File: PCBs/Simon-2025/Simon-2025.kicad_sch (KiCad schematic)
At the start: 13 parts, among them IC1 MSPM0G3507SDGS28R, J1 Conn_01x09, J2 Conn_01x05, SW6 SW_SPDT, U1 LIS2HH12

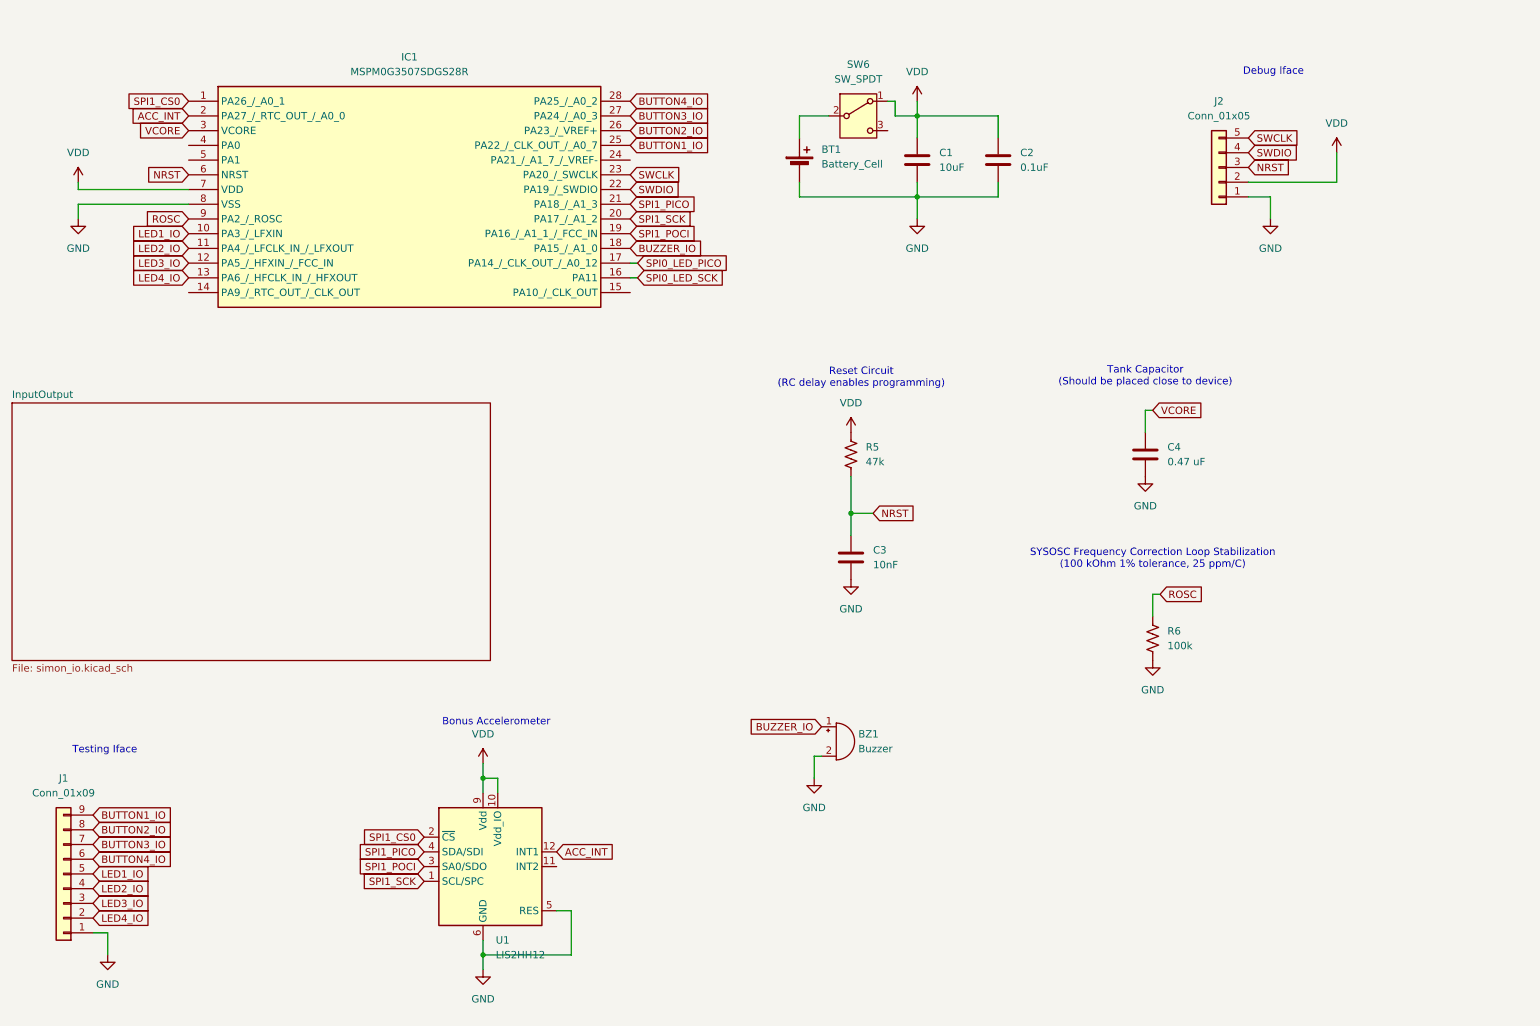
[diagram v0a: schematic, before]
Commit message: Updated Simon PCB 2025
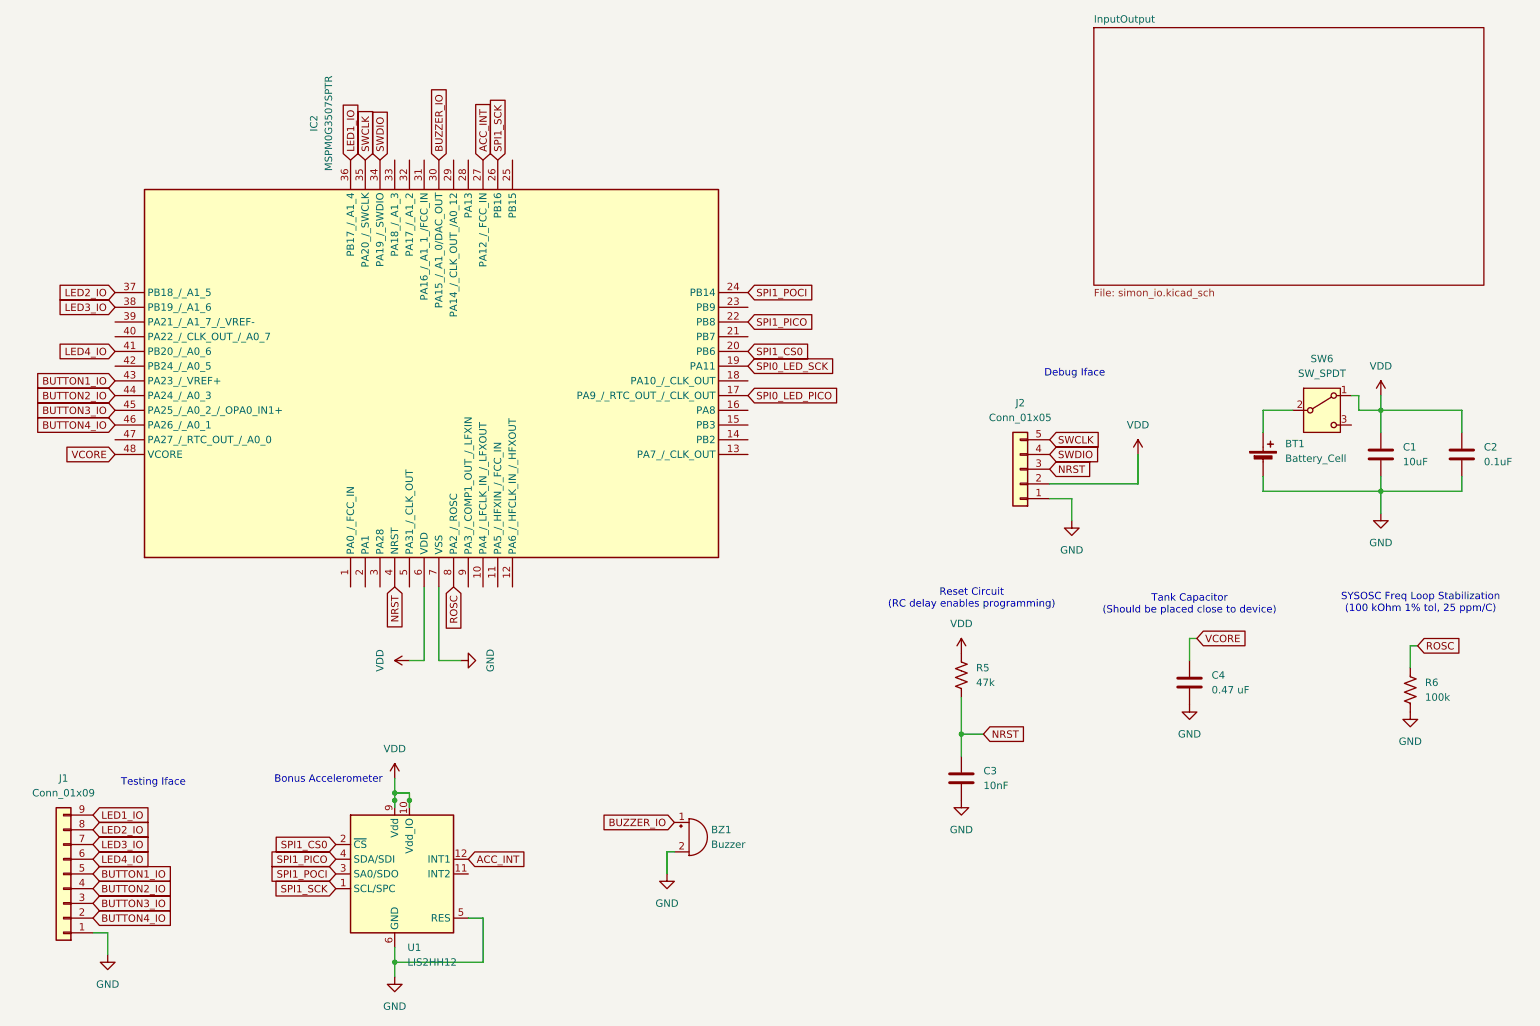
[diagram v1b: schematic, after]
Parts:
- removed IC1: MSPM0G3507SDGS28R, SOP50P490X110-28N, symbol ELEC327-Kicad:MSPM0G3507SDGS28R
- added IC2: MSPM0G3507SPTR, QFP50P900X900X160-48N, symbol ELEC327-Kicad:MSPM0G3507SPTR
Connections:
- net ACC_INT: now also IC2.27 (PA12_/_FCC_IN)
- net BUTTON1_IO: now also J1.5 (Pin_5), IC2.43 (PA23_/_VREF+); no longer J1.9 (Pin_9)
- net BUTTON2_IO: now also J1.4 (Pin_4), IC2.44 (PA24_/_A0_3); no longer J1.8 (Pin_8)
- net BUTTON3_IO: now also J1.3 (Pin_3), IC2.45 (PA25_/_A0_2_/_OPA0_IN1+); no longer J1.7 (Pin_7)
- net BUTTON4_IO: now also J1.2 (Pin_2), IC2.46 (PA26_/_A0_1); no longer J1.6 (Pin_6)
- net BUZZER_IO: now also IC2.30 (PA15_/_A1_0/DAC_OUT)
- net GND: now also IC2.7 (VSS)
- net LED1_IO: now also J1.9 (Pin_9), IC2.36 (PB17_/_A1_4); no longer J1.5 (Pin_5)
- net LED2_IO: now also J1.8 (Pin_8), IC2.37 (PB18_/_A1_5); no longer J1.4 (Pin_4)
- net LED3_IO: now also J1.7 (Pin_7), IC2.38 (PB19_/_A1_6); no longer J1.3 (Pin_3)
- net LED4_IO: now also J1.6 (Pin_6), IC2.41 (PB20_/_A0_6); no longer J1.2 (Pin_2)
- net NRST: now also IC2.4 (NRST)
- net ROSC: now also IC2.8 (PA2_/_ROSC)
- net SPI0_LED_PICO: now also IC2.17 (PA9_/_RTC_OUT_/_CLK_OUT)
- net SPI0_LED_SCK: now also IC2.19 (PA11)
- net SPI1_CS0: now also IC2.20 (PB6)
- net SPI1_PICO: now also IC2.22 (PB8)
- net SPI1_POCI: now also IC2.24 (PB14)
- net SPI1_SCK: now also IC2.26 (PB16)
- net SWCLK: now also IC2.35 (PA20_/_SWCLK)
- net SWDIO: now also IC2.34 (PA19_/_SWDIO)
- net VCORE: now also IC2.48 (VCORE)
- net VDD: now also IC2.6 (VDD)
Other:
- note added: "SYSOSC Freq Loop Stabilization (100 kOhm 1% tol, 25 ppm/C)"
- note removed: "SYSOSC Frequency Correction Loop Stabilization (100 kOhm 1% tolerance, 25 ppm/C)"
- moved on the sheet: BT1, BZ1, C1, C2, C3, C4, J2, R5, R6, SW6, U1
